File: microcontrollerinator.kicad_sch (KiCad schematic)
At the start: 46 parts, among them J1 USB_C_Receptacle_USB2.0_14P, J2 Conn_01x20, J3 Conn_01x20, J4 Conn_01x03, J5 Conn_01x03, Q1 AO3401A, SW1 SW_Push, U1 RP2040, U2 MCP1700x-330xxTT, U3 W25Q128JVS, U4 BQ21040DBV, Y1 12MHz

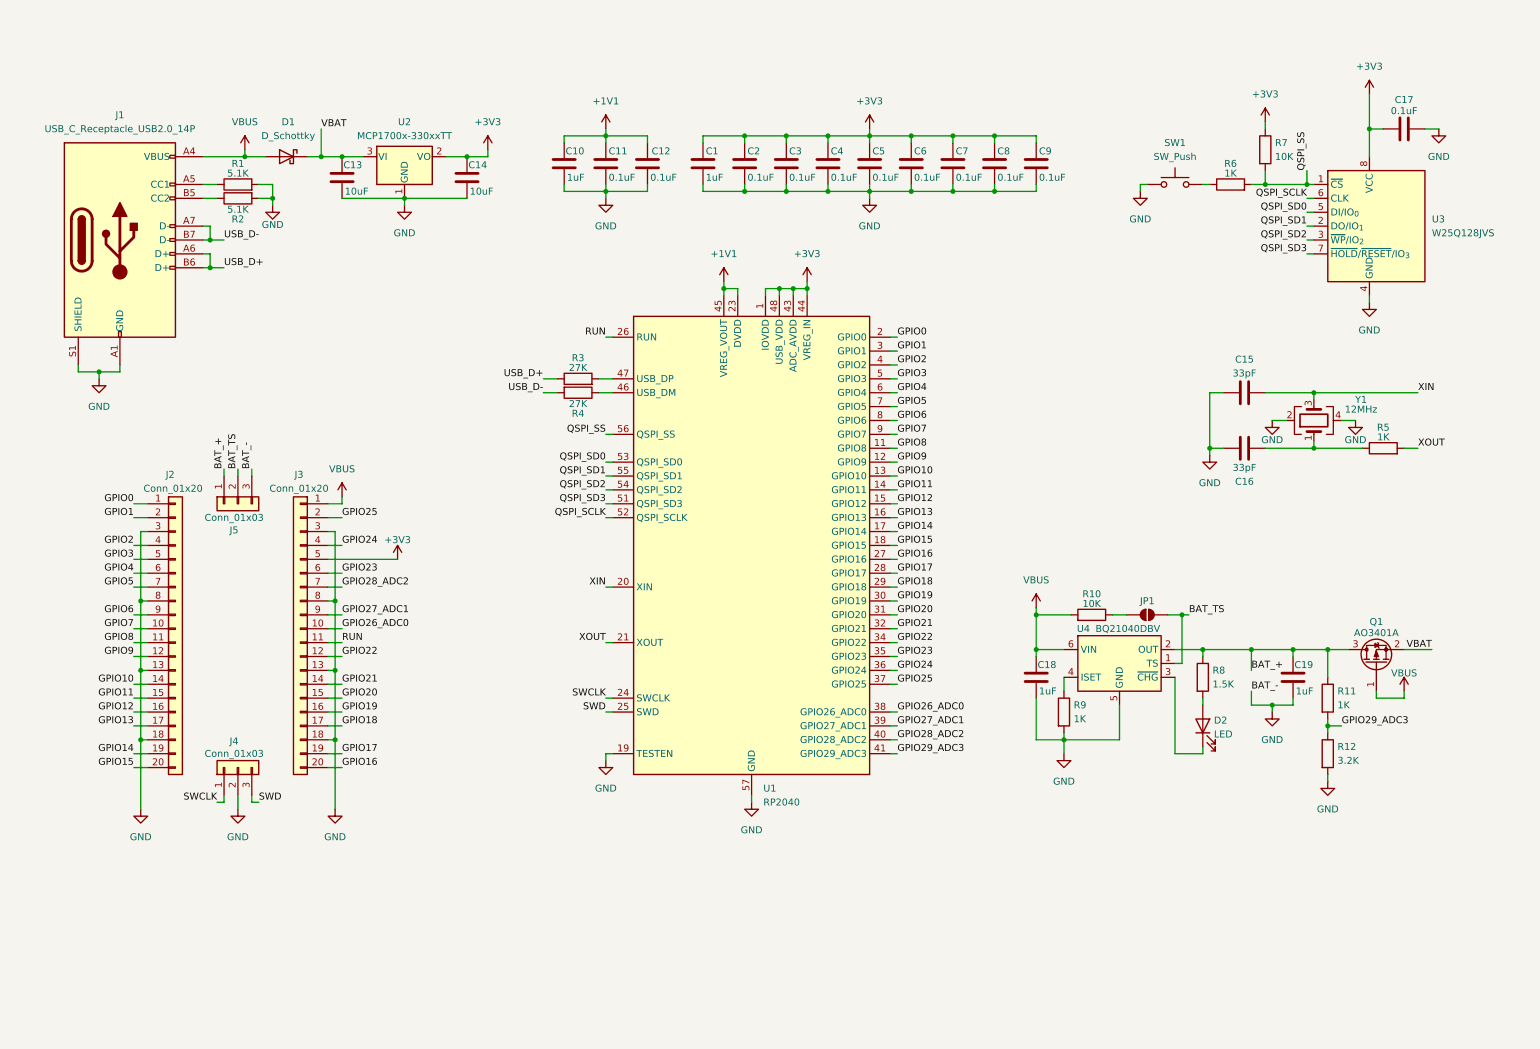
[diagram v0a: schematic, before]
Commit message: finished board
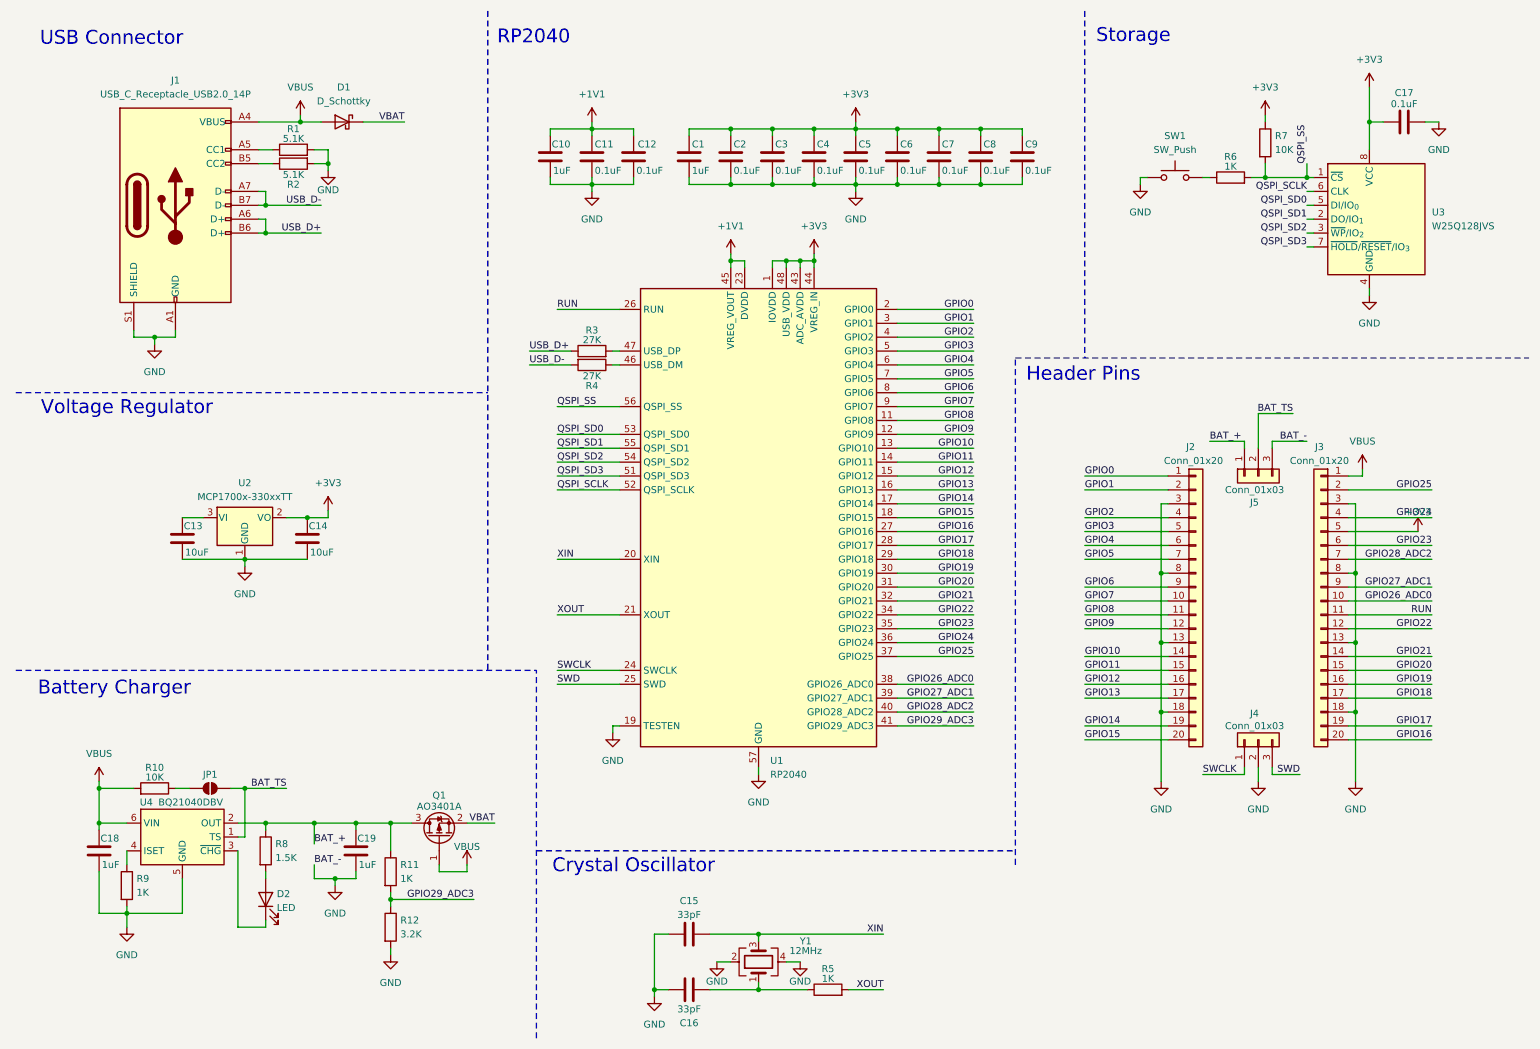
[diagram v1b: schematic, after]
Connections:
- net VBAT: no longer C13.1, U2.3 (VI)
- new net: C13.1, U2.3 (VI)
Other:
- note added: "Battery Charger"
- note added: "Crystal Oscillator"
- note added: "Header Pins"
- note added: "RP2040"
- note added: "Storage"
- note added: "USB Connector"
- note added: "Voltage Regulator"
- moved on the sheet: C1, C10, C11, C12, C13, C14, C15, C16, C17, C18, C19, C2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
